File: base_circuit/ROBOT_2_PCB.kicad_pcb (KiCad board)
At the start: 2 copper layers, 20 parts, among them J1 Conn_01x04, J2 Output_Supply, J3 Conn_01x01_Female, J4 M1,2, J5 M3,4, M1 Conn_01x04_Female, M2 Conn_01x04_Female, M3 Conn_01x04_Female, M4 Conn_01x04_Female, SW2 SW_SPDT

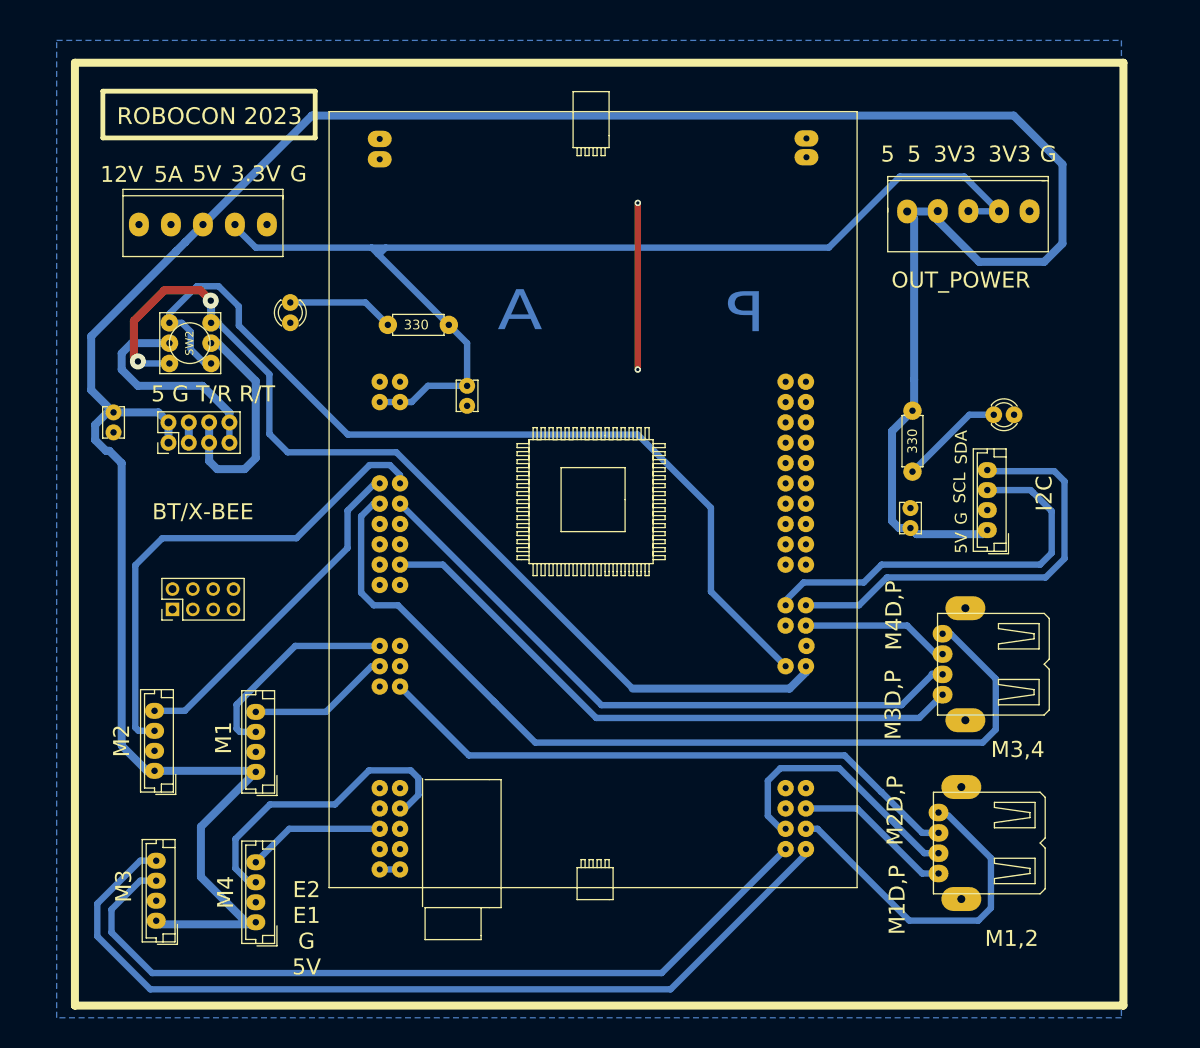
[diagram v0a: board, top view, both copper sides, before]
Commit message: Final design and add Pin Hole Size in  driLL_siZE.txt file
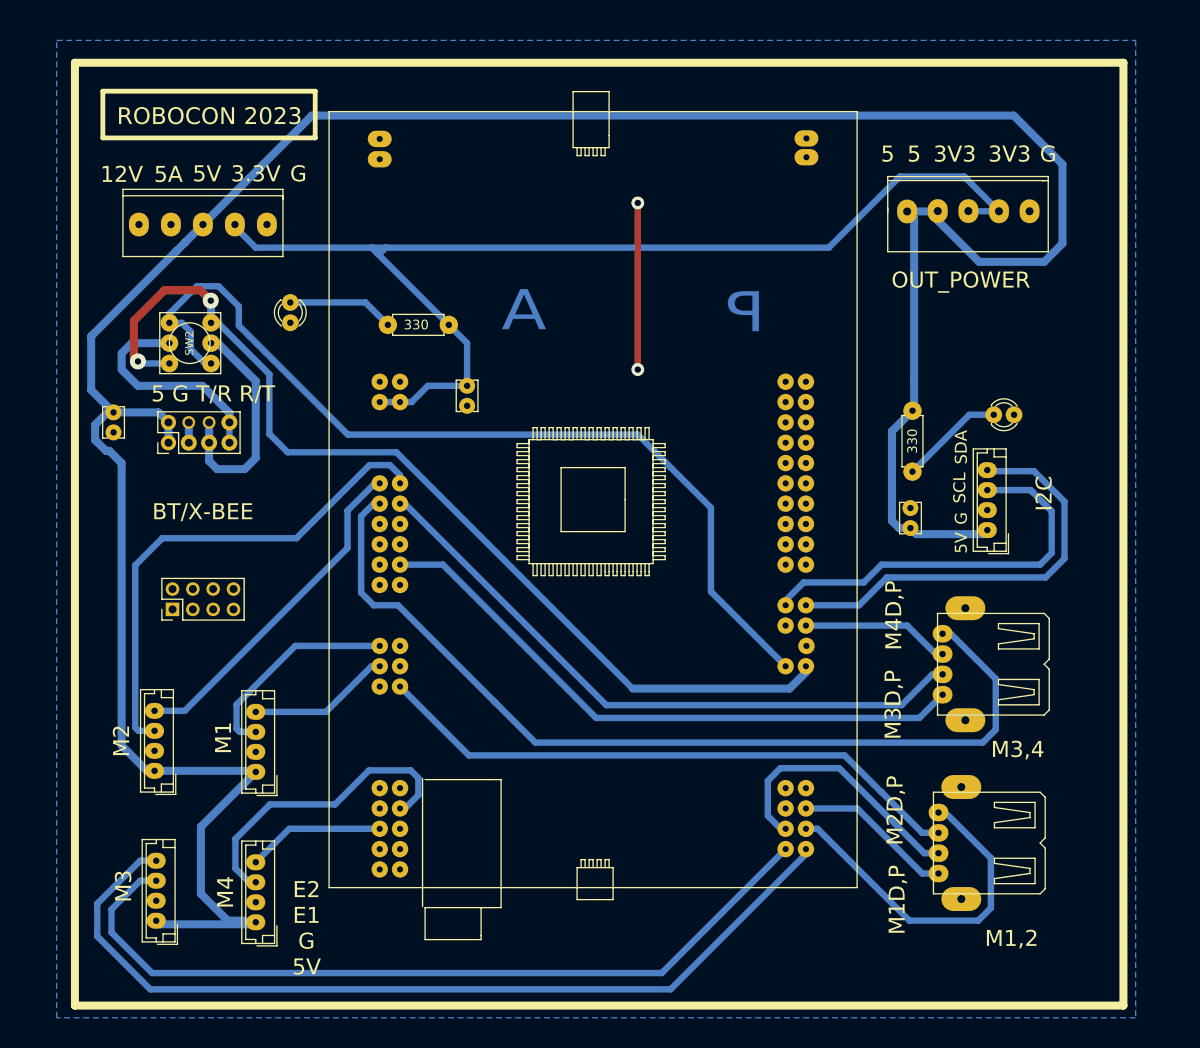
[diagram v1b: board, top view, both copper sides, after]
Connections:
- J1 pad 1: Net-(J1-Pad1) -> 5V
- J1 pad 2: Net-(J1-Pad2) -> 5V
- J1 pad 4: 5V -> GND
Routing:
- net unconnected-(S1-Pad50): track 2.54 -> 0.00 mm
- net SDA: track 54.6 -> 53.1 mm
- net 5V: track 342.4 -> 343.6 mm

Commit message: Final Edit of base circuit
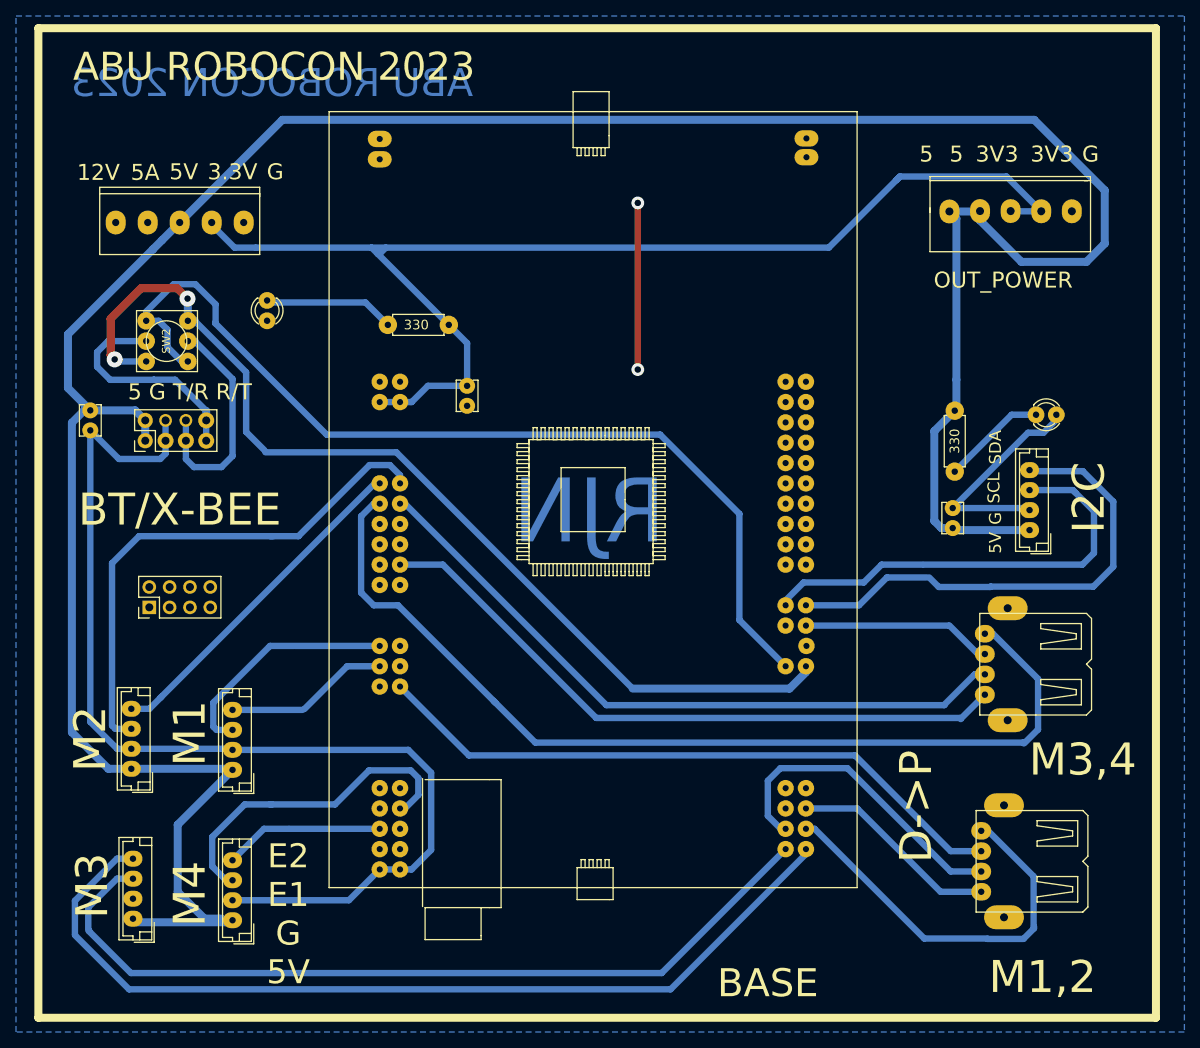
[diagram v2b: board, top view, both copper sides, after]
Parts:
- moved J4 5.80 mm to (158.5, 143.8)
- moved C2 5.28 mm to (148.6, 102.1)
- moved IMU1 5.28 mm to (158.2, 102.4)
- moved J5 5.28 mm to (159.0, 119.1)
- moved D3 5.28 mm to (159.0, 87.9)
- moved J2 5.28 mm to (150.8, 62.5)
- moved MPU1 5.28 mm to (148.8, 87.4)
- moved M2 2.92 mm to (45.9, 132.2)
- moved C3 2.92 mm to (40.8, 87.4)
- moved D2 2.92 mm to (62.9, 73.7)
- moved POW_SPLY1 2.92 mm to (47.0, 63.9)
- moved SW2 2.92 mm to (50.4, 78.7)
- moved J1 2.92 mm to (47.7, 91.2)
- moved J3 2.92 mm to (48.2, 112.0)
- moved M1 2.92 mm to (58.6, 132.3)
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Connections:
- S1 pad 50: unconnected-(S1-Pad50) -> GND
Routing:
- net GND: track 23.4 -> 182.8 mm
- net 3.3V: track 141.9 -> 150.9 mm
- net SDA: track 53.1 -> 61.3 mm
- net Motor_2_Pwm: track 42.3 -> 50.2 mm
- net M2D: track 74.9 -> 81.2 mm
- net M1D: track 19.9 -> 26.2 mm
- net Motor_1_Pwm: track 33.7 -> 39.9 mm
- net 5V: track 343.6 -> 349.5 mm
- net Motor_3_Pwm: track 79.8 -> 85.2 mm
- net M3D: track 77.0 -> 82.2 mm
- net Motor_4_Pwm: track 116.0 -> 121.2 mm
- net M4D: track 18.6 -> 23.7 mm
- net SCL: track 50.9 -> 56.0 mm
- net TX: track 115.4 -> 120.2 mm
- net Motor_2_Enc_1: track 62.9 -> 66.1 mm
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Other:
- board text added: "ABU ROBOCON 2023"
- board text added: "BASE"
- board text added: "D->P"
- board text added: "RJN"
- board text removed: "A"
- board text removed: "M1D,P"
- board text removed: "M2D,P"
- board text removed: "M3D,P"
- board text removed: "M4D,P"
- board text removed: "P"
- board text removed: "ROBOCON 2023"
